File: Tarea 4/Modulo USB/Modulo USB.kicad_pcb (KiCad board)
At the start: 2 copper layers, 2 parts, among them J1 USB_C_Receptacle_USB2.0_14P, J2 USB_C_Receptacle_USB2.0_14P

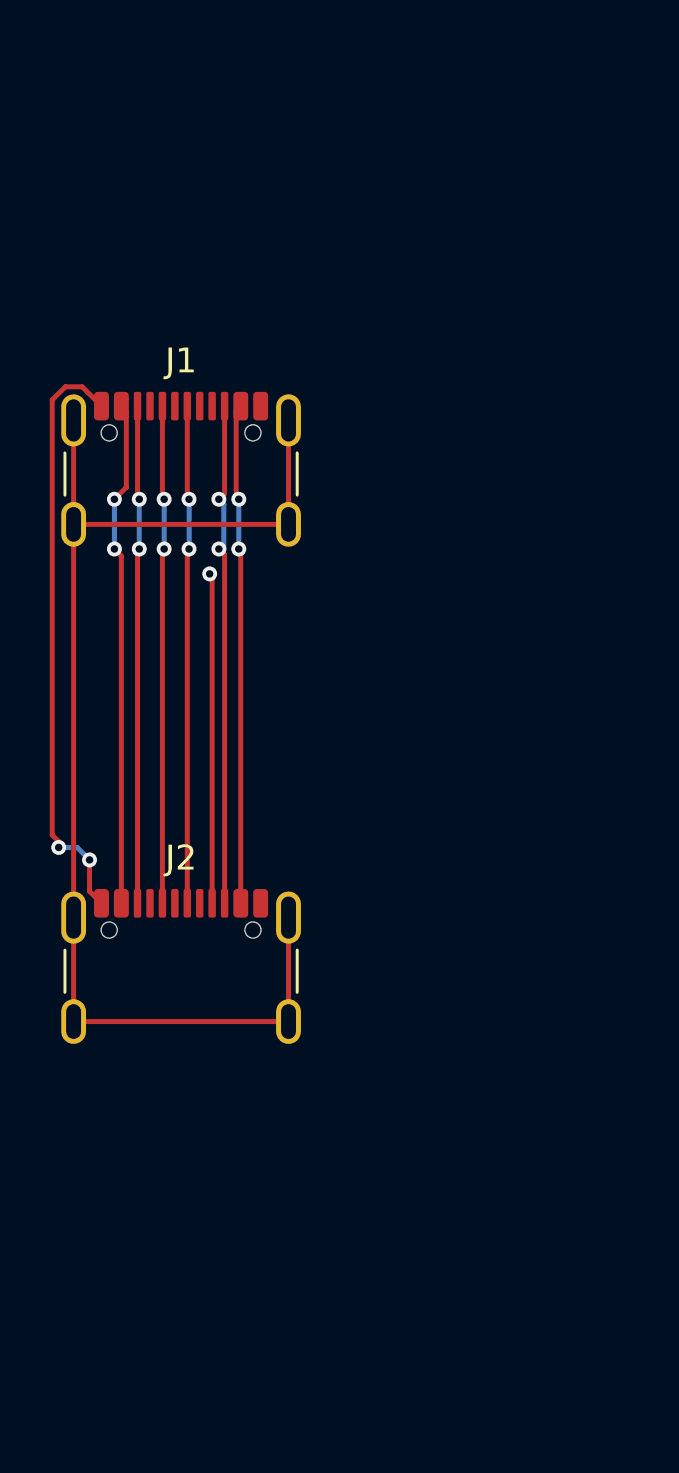
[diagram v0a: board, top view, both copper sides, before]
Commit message: Tarea 4
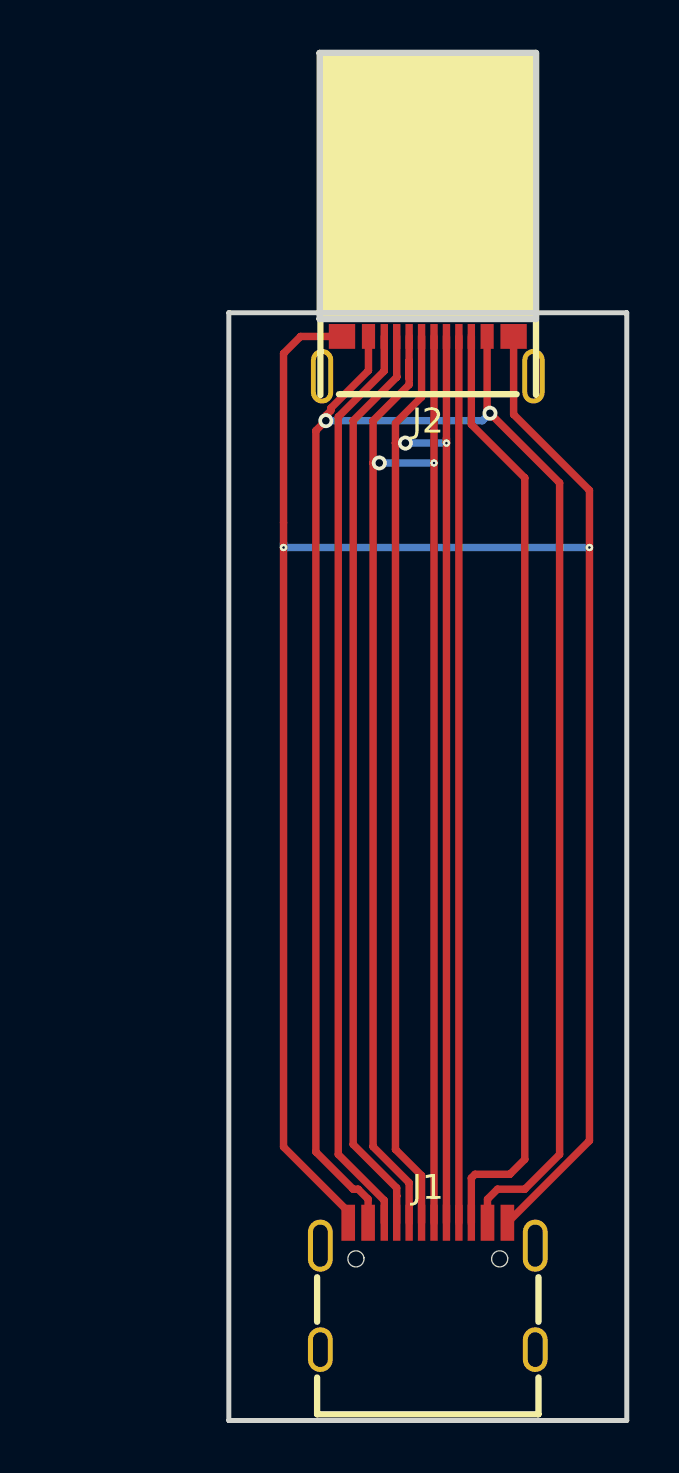
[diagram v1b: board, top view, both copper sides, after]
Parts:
- J1: footprint Connector_USB:USB_C_Receptacle_GCT_USB4105-xx-A_16P_TopMnt_Horizontal -> usb c male:USB-C-SMD_TYPE-C16PIN-SHOUHAN
- J2: footprint Connector_USB:USB_C_Receptacle_GCT_USB4105-xx-A_16P_TopMnt_Horizontal -> usb c male:USB-C-SMD_USBC1-AM-063
- moved J1 33.2 mm to (136.1, 118.6)
- moved J2 27.5 mm to (136.1, 81.3), turned to 180 degrees
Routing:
- net (no net): track 33.3 -> 245.3 mm, vias 3 -> 4
- net Net-(J1-D+-PadA6): track 0.00 -> 74.9 mm, vias 0 -> 2
- net Net-(J1-SHIELD): track 49.8 -> 0.00 mm
- net Net-(J1-VBUS-PadA4): track 40.5 -> 0.00 mm, vias 4 -> 0
- net Net-(J1-CC1): track 0.00 -> 37.1 mm
- net Net-(J1-D--PadA7): track 40.1 -> 75.9 mm, vias 4 -> 2
- net Net-(J1-GND-PadA1): track 24.0 -> 0.00 mm, vias 2 -> 0
- net Net-(J1-CC2): track 20.5 -> 38.2 mm, vias 2 -> 0
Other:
- board outline added: 16 x 44.5 mm
- copper layers 2 -> 4
